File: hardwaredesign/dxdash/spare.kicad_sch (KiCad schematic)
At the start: 6 parts, among them J10 Screw_Terminal_01x04, J11 Screw_Terminal_01x04, J13 Conn_01x01_Pin, J3 Screw_Terminal_01x04, J7 Screw_Terminal_01x04, J9 Screw_Terminal_01x04

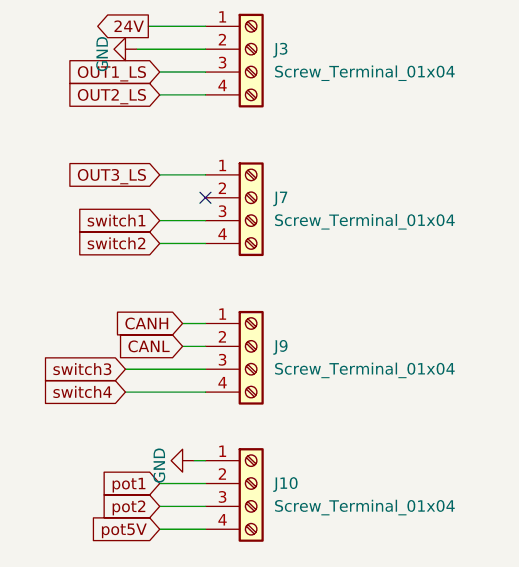
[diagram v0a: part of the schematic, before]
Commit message: more layout
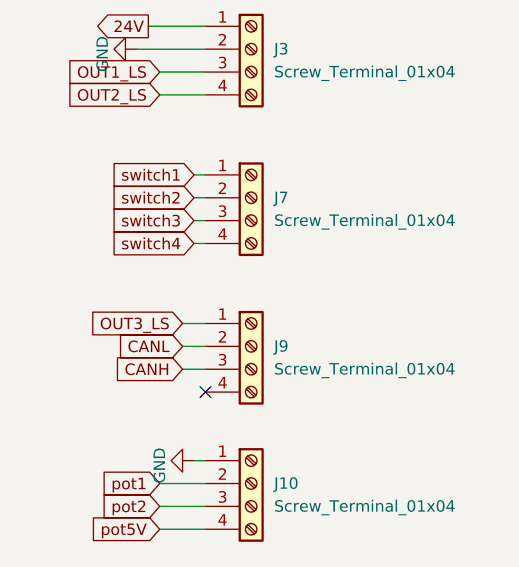
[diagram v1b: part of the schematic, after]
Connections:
- net CANH: now also J9.3 (Pin_3); no longer J9.1 (Pin_1)
- net OUT3_LS: now also J9.1 (Pin_1); no longer J7.1 (Pin_1)
- net switch1: now also J7.1 (Pin_1); no longer J7.3 (Pin_3)
- net switch2: now also J7.2 (Pin_2); no longer J7.4 (Pin_4)
- net switch3: now also J7.3 (Pin_3); no longer J9.3 (Pin_3)
- net switch4: now also J7.4 (Pin_4); no longer J9.4 (Pin_4)
